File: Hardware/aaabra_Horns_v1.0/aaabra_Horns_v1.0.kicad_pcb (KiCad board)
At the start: 2 copper layers, 0 parts

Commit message: Finished pcb for horns
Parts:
- added C1: .1u, Capacitor_SMD:C_0805_2012Metric, F.Cu at (131.8, 103.8)
- added C2: .1u, Capacitor_SMD:C_0805_2012Metric, F.Cu at (135.8, 114.0)
- added C3: .1u, Capacitor_SMD:C_0805_2012Metric, F.Cu at (139.3, 114.0)
- added C4: .1u, Capacitor_SMD:C_0805_2012Metric, F.Cu at (142.7, 115.8)
- added C5: 1u, Capacitor_SMD:C_0805_2012Metric, F.Cu at (146.3, 115.8)
- added C6: 1u, Capacitor_SMD:C_0805_2012Metric, F.Cu at (149.0, 104.2)
- added C7: 10u, Capacitor_SMD:C_0805_2012Metric, F.Cu at (142.4, 107.6)
- added C8: 10u, Capacitor_SMD:C_0805_2012Metric, F.Cu at (142.4, 111.1)
- added C9: 100u, Capacitor_THT:CP_Radial_D5.0mm_P2.00mm, F.Cu at (134.4, 96.5)
- added D1: ES2DA, Diode_SMD:D_SMA, F.Cu at (137.6, 104.1)
- added F1: 2, Fuse:Fuse_1206_3216Metric_Pad1.42x1.75mm_HandSolder, F.Cu at (139.9, 96.0)
- added J1: Conn_01x03, Connector_Molex:Molex_KK-254_AE-6410-03A_1x03_P2.54mm_Vertical, F.Cu at (146.8, 112.8)
- added J2: Conn_01x02, Connector_Molex:Molex_KK-254_AE-6410-02A_1x02_P2.54mm_Vertical, F.Cu at (125.5, 103.5)
- added J3: Conn_01x02, Connector_Molex:Molex_KK-254_AE-6410-02A_1x02_P2.54mm_Vertical, F.Cu at (144.6, 95.3)
- added J4: Conn_01x02, Connector_Molex:Molex_KK-254_AE-6410-02A_1x02_P2.54mm_Vertical, F.Cu at (144.6, 101.5)
- added Q1: IRFR010PBF, Package_TO_SOT_SMD:TO-252-2, F.Cu at (135.6, 109.5)
- added R1: 1k, Resistor_SMD:R_0603_1608Metric_Pad0.98x0.95mm_HandSolder, F.Cu at (131.8, 101.0)
- added REF**: MountingHole_2.1mm, MountingHole:MountingHole_2.1mm, F.Cu at (125.7, 115.6)
- added REF**: MountingHole_2.1mm, MountingHole:MountingHole_2.1mm, F.Cu at (152.4, 94.2)
- added REF**: MountingHole_2.1mm, MountingHole:MountingHole_2.1mm, F.Cu at (152.4, 115.6)
- added REF**: MountingHole_2.1mm, MountingHole:MountingHole_2.1mm, F.Cu at (125.8, 94.2)
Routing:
- net +24V: track 0.00 -> 104.9 mm
- net GND: track 0.00 -> 79.4 mm
- net /Horn_In: track 0.00 -> 14.2 mm
- net /HORN_CTL: track 0.00 -> 11.8 mm
- net Net-(J3-Pin_1): track 0.00 -> 5.52 mm
- net Net-(J3-Pin_2): track 0.00 -> 3.70 mm
- added copper zone on F.Cu, net +24V
- added copper zone on B.Cu, net GND
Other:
- board outline added: 31.8 x 26.4 mm

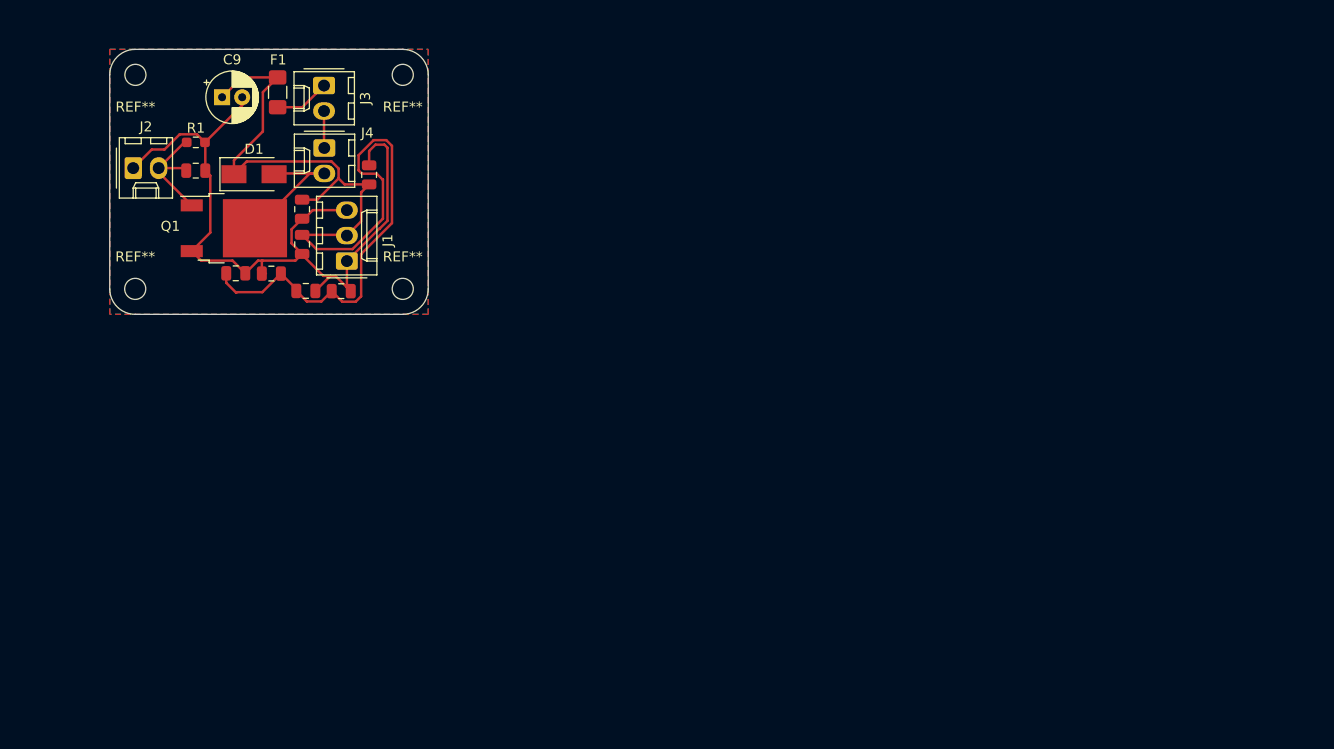
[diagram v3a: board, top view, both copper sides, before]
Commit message: onboarding
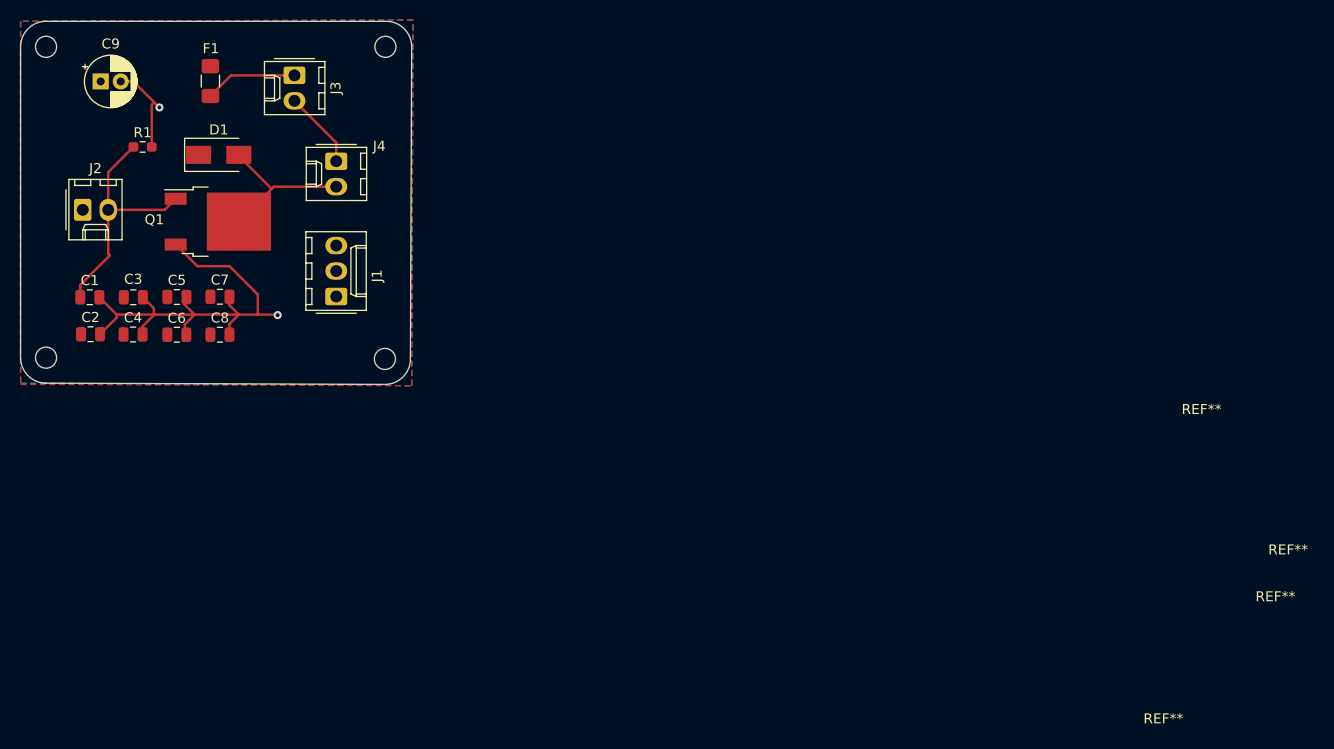
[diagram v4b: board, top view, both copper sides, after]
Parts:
- moved C6 24.9 mm to (129.9, 120.1), turned to 0 degrees
- moved C4 17.8 mm to (125.5, 120.1)
- moved C1 16.5 mm to (121.2, 116.4)
- moved C5 16.4 mm to (129.9, 116.4)
- moved C2 15.7 mm to (121.3, 120.1)
- moved C3 14.0 mm to (125.5, 116.4), turned to 0 degrees
- moved C9 12.2 mm to (122.3, 94.9)
- moved C8 12.2 mm to (134.2, 120.1), turned to 0 degrees
- moved C7 12.0 mm to (134.2, 116.4), turned to 0 degrees
- moved REF** 11.2 mm to (116.8, 122.4)
- moved REF** 9.34 mm to (116.8, 91.4)
- moved REF** 7.21 mm to (150.6, 122.6)
- moved F1 6.80 mm to (133.2, 94.9)
- moved J2 6.53 mm to (120.5, 107.7)
- moved R1 5.33 mm to (126.5, 101.4)
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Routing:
- net +24V: track 104.9 -> 0.00 mm
- net GND: track 79.4 -> 56.7 mm, vias 0 -> 2
- net /HORN_CTL: track 11.8 -> 24.5 mm
- net /Horn_In: track 14.2 -> 18.4 mm
- net Net-(J3-Pin_2): track 3.70 -> 7.75 mm
- net Net-(J3-Pin_1): track 5.52 -> 9.23 mm
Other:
- board size 31.8 x 26.4 mm -> 39 x 36.2 mm
